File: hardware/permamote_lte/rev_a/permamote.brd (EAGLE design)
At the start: 27 x 60 mm, 119 parts, among them IC1 NRF9160, J1 TC2030-JLINK-NL, J2 U.FL-R-SMT, J3 NANO_SIM, J4 U.FL-R-SMT, J5 DM3AT-SF-PEJM5, Q1 PMDXB950UPEL, Q10 PMDXB950UPEL, Q2 PMDXB950UPEL, Q3 PMDXB950UPEL, Q4 PMDXB950UPEL, Q5 PMDXB950UPEL, Q6 PMDXB950UPEL, Q7 PMDXB950UPEL, Q8 PMDXB950UPEL, U1 AB1815-T3, U10 SIP32510, U11 SI7021-A20-GM1, U12 TCS34725, U2 BQ25505, U3 EKMB1101111, U4 BGA725L6, U5 TPD3F303DPVR, U6 LIS2DW12, U7 MAX17222, U8 MAX44009, U9 MS5637-02BA03, X4 ABS07-32.768KHZ-7-T

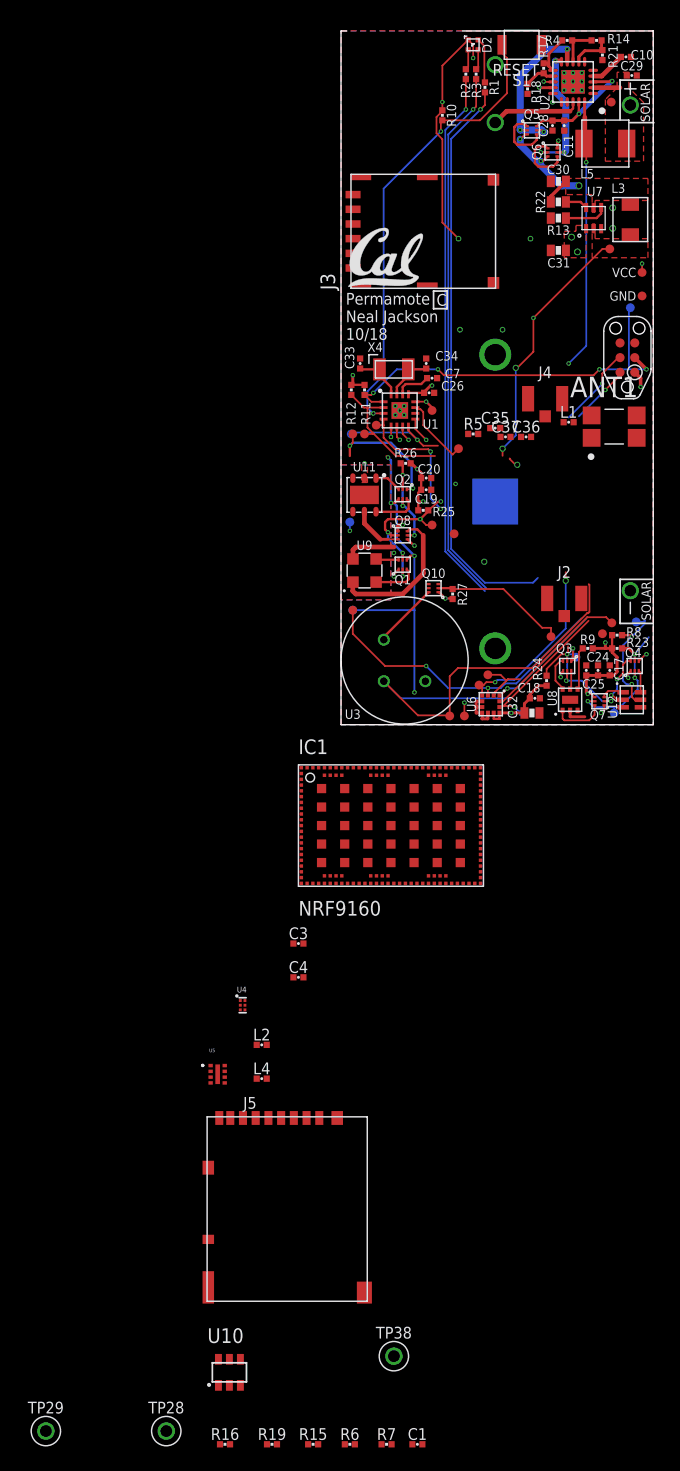
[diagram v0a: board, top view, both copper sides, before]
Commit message: layout
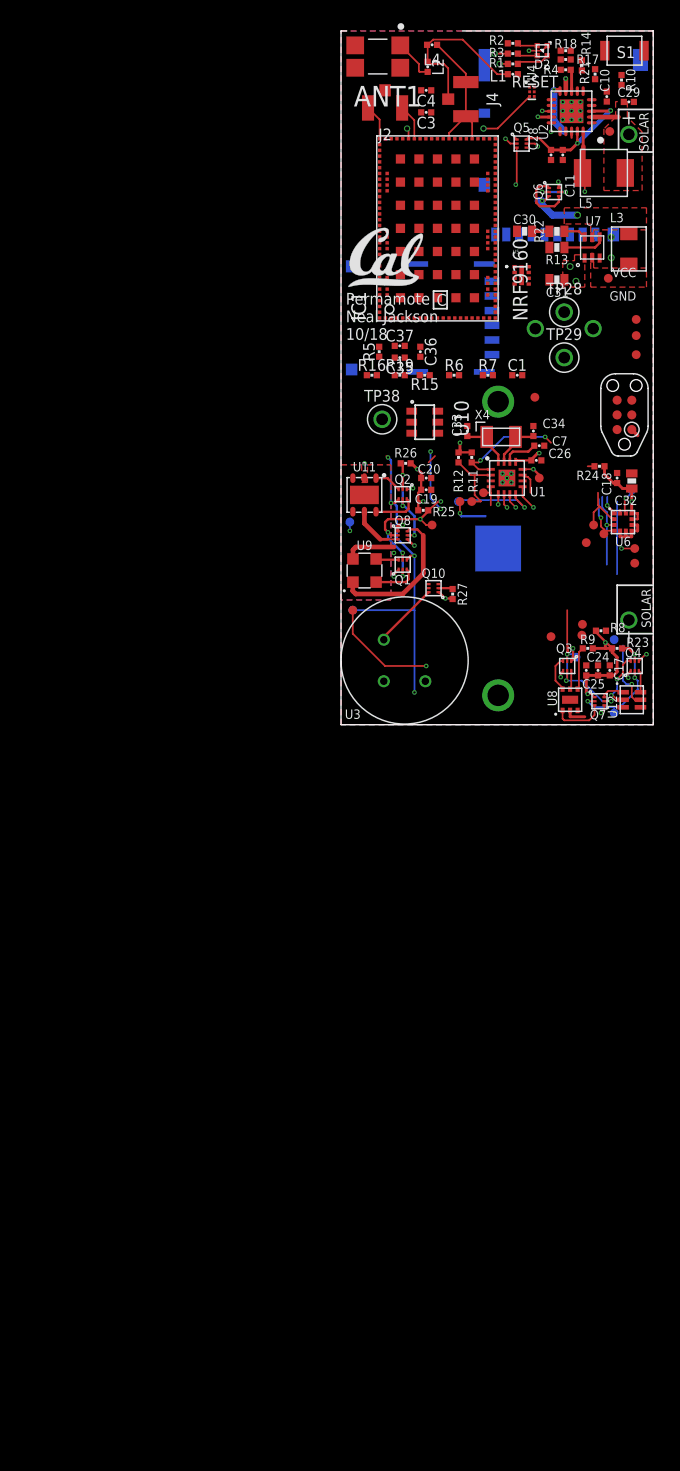
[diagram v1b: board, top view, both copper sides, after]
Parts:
- moved TP29 103.1 mm to (19.3, 31.8)
- moved TP28 102.7 mm to (19.3, 35.7)
- moved R16 93.3 mm to (2.67, 30.2)
- moved R19 93.1 mm to (5.08, 30.2)
- moved R15 93.0 mm to (7.24, 30.2), turned to 180 degrees
- moved R6 92.9 mm to (9.78, 30.2)
- moved R7 92.9 mm to (12.7, 30.2)
- moved C1 92.9 mm to (15.2, 30.2)
- moved L4 90.6 mm to (7.87, 58.8), turned to 180 degrees
- moved L2 85.8 mm to (7.49, 56.9), turned to 270 degrees
- moved U10 83.9 mm to (7.24, 26.2), turned to 270 degrees
- moved U4 82.9 mm to (16.5, 54.7)
- moved TP38 81.0 mm to (3.56, 26.4)
- moved J5 79.9 mm to (18.8, 42.3), flipped to the bottom, turned to 180 degrees
- moved C4 77.5 mm to (7.37, 54.9), turned to 180 degrees
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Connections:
- removed net DBG_RX: IC1.P0.30
- removed net DBG_TX: IC1.P0.31
- net !LT_EN: now also IC1.P0.30; no longer IC1.P0.09
- net !RTC_IRQ3: now also IC1.P0.09
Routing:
- net LED_GREEN: track 46.4 -> 0.00 mm, vias 1 -> 0
- net LED_RED: track 49.6 -> 3.63 mm
- net SCL: track 65.0 -> 21.1 mm, vias 6 -> 5
- net LED_BLUE: track 46.4 -> 5.18 mm
- net VSEC: track 41.3 -> 0.55 mm, vias 1 -> 0
- net !RTC_EXTR: track 40.1 -> 0.18 mm, vias 2 -> 0
- net VSOL: track 47.2 -> 12.3 mm, vias 1 -> 0
- net MOSI: track 43.5 -> 9.00 mm, vias 3 -> 2
- net VBAT: track 44.7 -> 11.0 mm
- net SCK: track 42.1 -> 8.80 mm
- net PIR_OUT: track 38.8 -> 6.35 mm
- net VCC: track 67.2 -> 35.0 mm, vias 21 -> 14
- net !RST: track 36.8 -> 9.88 mm, vias 4 -> 2
- net VBAT_OK: track 28.7 -> 3.18 mm
- net SW: track 22.2 -> 0.00 mm, vias 3 -> 0
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- removed copper zone on layer 15, net VBAT
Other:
- board text removed: "CR123A PACK +"
